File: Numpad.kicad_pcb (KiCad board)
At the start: 2 copper layers, 94 x 162.6 mm, 68 parts, among them J1 SWD, J2 USB_C_Receptacle_USB2.0, SW1 SW_Push, SW10 SW_Push, SW11 SW_Push, SW12 SW_Push, SW13 SW_Push, SW14 SW_Push, SW15 SW_Push, SW16 SW_Push, SW17 SW_Push, SW18 SW_Push, SW19 SW_Push, SW2 SW_Push, SW20 SW_Push, SW21 SW_Push, SW3 SW_Push, SW4 SW_Push, SW5 SW_Push, SW6 SW_Push, SW7 SW_Push, SW8 SW_Push, SW9 SW_Push, U1 SRV05-4, U2 STM32F103C8Tx, U3 XC6206PxxxMR, Y1 8MHz

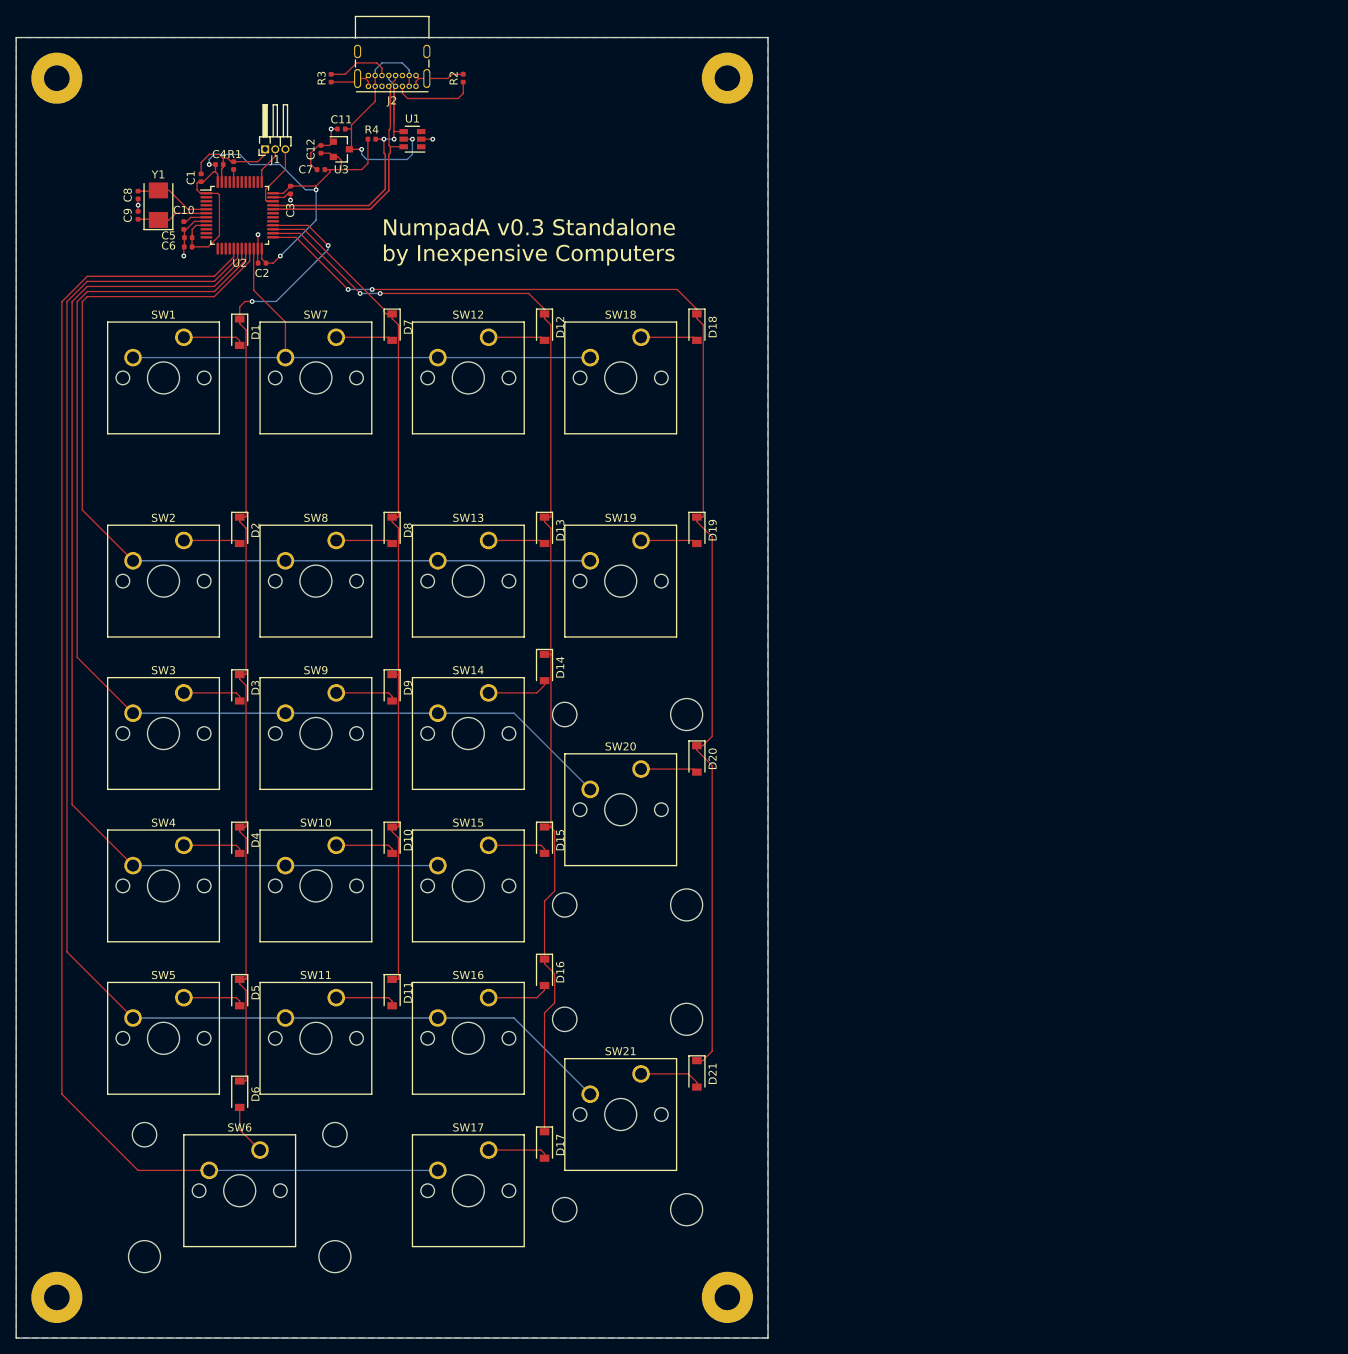
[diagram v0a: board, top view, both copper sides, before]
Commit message: v0.4
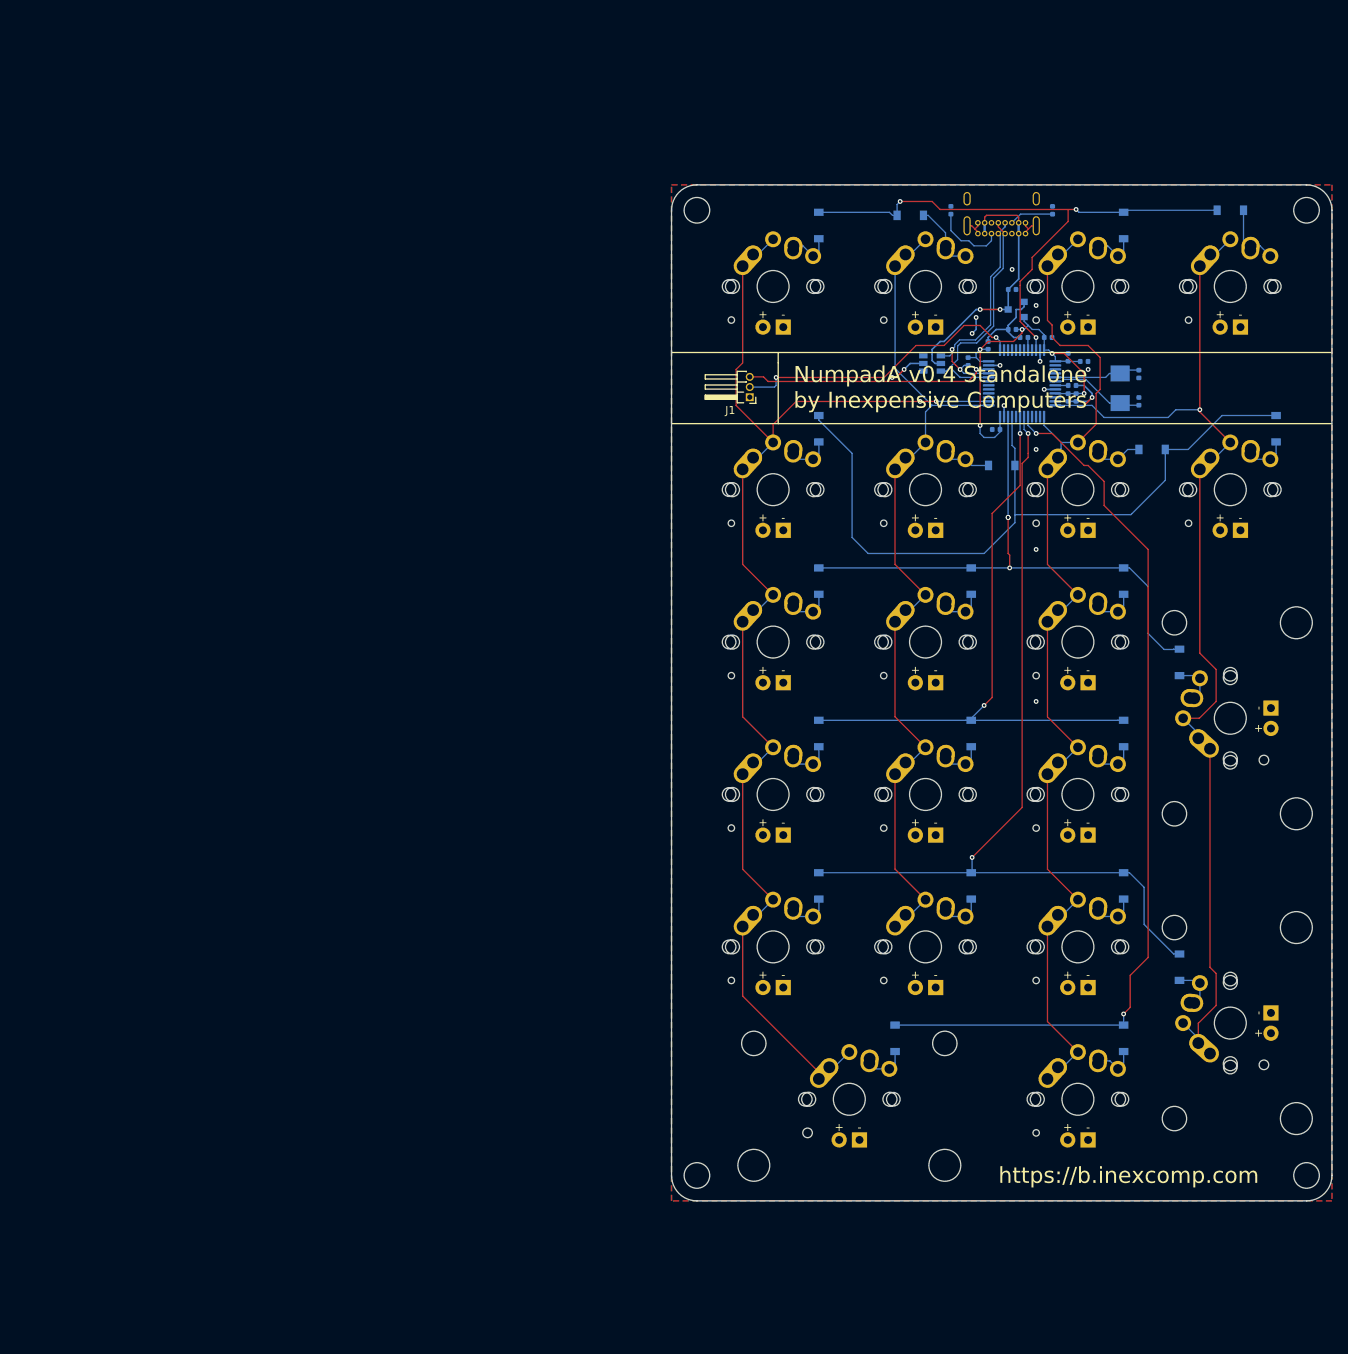
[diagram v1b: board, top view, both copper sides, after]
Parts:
- removed D1, D10, D11, D12, D13, D14, D15, D16, D17, D18, D19, D2, D20, D21, D3, D4, D5, D6, D7, D8, D9: 1N4148, Diode_SMD:D_SOD-123
- removed SW1, SW10, SW11, SW12, SW13, SW14, SW15, SW16, SW17, SW18, SW19, SW2, SW3, SW4, SW5, SW7, SW8, SW9: SW_Push, Button_Switch_Keyboard:SW_Cherry_MX_1.00u_PCB
- removed SW20, SW21: SW_Push, Button_Switch_Keyboard:SW_Cherry_MX_2.00u_Vertical_PCB
- removed SW6: SW_Push, Button_Switch_Keyboard:SW_Cherry_MX_2.00u_PCB
- added D_0: 1N4148, Diode_SMD:D_SOD-123, B.Cu at (126.4, 141.6)
- added D_1: 1N4148, Diode_SMD:D_SOD-123, B.Cu at (116.8, 122.6)
- added D_2: 1N4148, Diode_SMD:D_SOD-123, B.Cu at (135.9, 122.6)
- added D_3: 1N4148, Diode_SMD:D_SOD-123, B.Cu at (154.9, 122.6)
- added D_4: 1N4148, Diode_SMD:D_SOD-123, B.Cu at (116.8, 103.5)
- added D_5: 1N4148, Diode_SMD:D_SOD-123, B.Cu at (135.9, 103.5)
- added D_6: 1N4148, Diode_SMD:D_SOD-123, B.Cu at (154.9, 103.5)
- added D_7: 1N4148, Diode_SMD:D_SOD-123, B.Cu at (116.8, 84.5)
- added D_8: 1N4148, Diode_SMD:D_SOD-123, B.Cu at (135.9, 84.5)
- added D_9: 1N4148, Diode_SMD:D_SOD-123, B.Cu at (154.9, 84.5)
- added D_BKSP1: 1N4148, Diode_SMD:D_SOD-123, B.Cu at (168.3, 38.1)
- added D_DOT1: 1N4148, Diode_SMD:D_SOD-123, B.Cu at (154.9, 141.6)
- added D_ENTER1: 1N4148, Diode_SMD:D_SOD-123, B.Cu at (161.9, 132.7)
- added D_ESC1: 1N4148, Diode_SMD:D_SOD-123, B.Cu at (116.8, 40.0)
- added D_FN1: 1N4148, Diode_SMD:D_SOD-123, B.Cu at (154.9, 40.0)
- added D_MINUS1: 1N4148, Diode_SMD:D_SOD-123, B.Cu at (174.0, 65.4)
- added D_NUMLK1: 1N4148, Diode_SMD:D_SOD-123, B.Cu at (116.8, 65.4)
- added D_PLUS1: 1N4148, Diode_SMD:D_SOD-123, B.Cu at (161.9, 94.6)
- added D_SLASH1: 1N4148, Diode_SMD:D_SOD-123, B.Cu at (139.7, 70.0)
- added D_STAR1: 1N4148, Diode_SMD:D_SOD-123, B.Cu at (158.5, 68.0)
- added D_TAB1: 1N4148, Diode_SMD:D_SOD-123, B.Cu at (128.3, 38.7)
- added SW_0: SW_Push, Keebio-Parts:MX-Alps-Choc-2U, F.Cu at (120.7, 149.2)
- added SW_1: SW_Push, Keebio-Parts:MX-Alps-Choc-1U, F.Cu at (111.1, 130.2)
- added SW_2: SW_Push, Keebio-Parts:MX-Alps-Choc-1U, F.Cu at (130.2, 130.2)
- added SW_3: SW_Push, Keebio-Parts:MX-Alps-Choc-1U, F.Cu at (149.2, 130.2)
- added SW_4: SW_Push, Keebio-Parts:MX-Alps-Choc-1U, F.Cu at (111.1, 111.1)
- added SW_5: SW_Push, Keebio-Parts:MX-Alps-Choc-1U, F.Cu at (130.2, 111.1)
- added SW_6: SW_Push, Keebio-Parts:MX-Alps-Choc-1U, F.Cu at (149.2, 111.1)
- added SW_7: SW_Push, Keebio-Parts:MX-Alps-Choc-1U, F.Cu at (111.1, 92.1)
- added SW_8: SW_Push, Keebio-Parts:MX-Alps-Choc-1U, F.Cu at (130.2, 92.1)
- added SW_9: SW_Push, Keebio-Parts:MX-Alps-Choc-1U, F.Cu at (149.2, 92.1)
- added SW_BKSP1: SW_Push, Keebio-Parts:MX-Alps-Choc-1U, F.Cu at (168.3, 47.6)
- added SW_DOT1: SW_Push, Keebio-Parts:MX-Alps-Choc-1U, F.Cu at (149.2, 149.2)
- added SW_ENTER1: SW_Push, Keebio-Parts:MX-Alps-Choc-2U, F.Cu at (168.3, 139.7)
- added SW_ESC1: SW_Push, Keebio-Parts:MX-Alps-Choc-1U, F.Cu at (111.1, 47.6)
- added SW_FN1: SW_Push, Keebio-Parts:MX-Alps-Choc-1U, F.Cu at (149.2, 47.6)
- added SW_MINUS1: SW_Push, Keebio-Parts:MX-Alps-Choc-1U, F.Cu at (168.3, 73.0)
- added SW_NUMLK1: SW_Push, Keebio-Parts:MX-Alps-Choc-1U, F.Cu at (111.1, 73.0)
- added SW_PLUS1: SW_Push, Keebio-Parts:MX-Alps-Choc-2U, F.Cu at (168.3, 101.6)
- added SW_SLASH1: SW_Push, Keebio-Parts:MX-Alps-Choc-1U, F.Cu at (130.2, 73.0)
- added SW_STAR1: SW_Push, Keebio-Parts:MX-Alps-Choc-1U, F.Cu at (149.2, 73.0)
- added SW_TAB1: SW_Push, Keebio-Parts:MX-Alps-Choc-1U, F.Cu at (130.2, 47.6)
- C1, C10, C11, C12, C2, C3, C4, C5, C6, C7, C8, C9, J2, R1, R2, R3, R4, U1, U2, U3, Y1: moved to B.Cu
- H1, H2, H3, H4: value MountingHole_Pad -> MountingHole; footprint MountingHole:MountingHole_3.2mm_M3_Pad -> MountingHole:MountingHole_3.2mm_M3
- moved C9 127.2 mm to (156.8, 62.0)
- moved C8 127.1 mm to (156.8, 58.6)
- moved Y1 122.4 mm to (154.5, 60.4)
- moved C10 112.8 mm to (148.5, 60.0), turned to 180 degrees
- moved C5 112.8 mm to (149.0, 61.5), turned to 90 degrees
- moved C6 111.6 mm to (148.0, 61.5), turned to 90 degrees
- moved C1 110.7 mm to (148.0, 56.5)
- moved C4 105.8 mm to (145.5, 54.0)
- moved R1 101.1 mm to (142.5, 54.0), turned to 180 degrees
- moved U2 100.0 mm to (142.2, 59.7), turned to 180 degrees
- moved C7 98.4 mm to (150.0, 57.0), turned to 180 degrees
- moved C2 94.1 mm to (139.0, 65.5)
- moved R3 91.7 mm to (146.1, 38.1), turned to 270 degrees
- moved C3 89.3 mm to (138.0, 55.0), turned to 270 degrees
- moved C12 89.3 mm to (141.0, 53.0), turned to 180 degrees
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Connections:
- H1 pad 1: GND -> (no net)
- H2 pad 1: GND -> (no net)
- H3 pad 1: GND -> (no net)
- H4 pad 1: GND -> (no net)
- J2 pad A8: Net-(J2-PadA8) -> (no net)
- J2 pad B8: Net-(J2-PadB8) -> (no net)
- U1 pad 1: Net-(U1-Pad1) -> (no net)
- U1 pad 3: Net-(U1-Pad3) -> (no net)
- U2 pad 10: Net-(U2-Pad10) -> (no net)
- U2 pad 11: Net-(U2-Pad11) -> (no net)
- U2 pad 12: Net-(U2-Pad12) -> col4
- U2 pad 13: Net-(U2-Pad13) -> col3
- U2 pad 14: Net-(U2-Pad14) -> (no net)
- U2 pad 15: Net-(U2-Pad15) -> (no net)
- U2 pad 16: Net-(U2-Pad16) -> (no net)
- U2 pad 2: Net-(U2-Pad2) -> (no net)
- U2 pad 20: row3 -> (no net)
- U2 pad 22: row1 -> row3
- U2 pad 25: col4 -> col2
- U2 pad 26: col3 -> col1
- U2 pad 27: col2 -> (no net)
- U2 pad 28: col1 -> (no net)
- U2 pad 29: Net-(U2-Pad29) -> (no net)
- U2 pad 3: Net-(U2-Pad3) -> (no net)
- U2 pad 30: Net-(U2-Pad30) -> (no net)
- U2 pad 31: Net-(U2-Pad31) -> (no net)
- U2 pad 38: Net-(U2-Pad38) -> (no net)
- U2 pad 39: Net-(U2-Pad39) -> (no net)
- U2 pad 4: Net-(U2-Pad4) -> (no net)
- U2 pad 40: Net-(U2-Pad40) -> (no net)
- U2 pad 41: Net-(U2-Pad41) -> (no net)
- U2 pad 42: Net-(U2-Pad42) -> (no net)
- U2 pad 43: Net-(U2-Pad43) -> (no net)
- U2 pad 45: Net-(U2-Pad45) -> (no net)
- U2 pad 46: Net-(U2-Pad46) -> row1
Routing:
- net row3: track 140.1 -> 71.8 mm, vias 0 -> 3
- net row5: track 178.8 -> 112.2 mm, vias 0 -> 2
- net row6: track 174.8 -> 113.6 mm, vias 0 -> 2
- net row4: track 136.5 -> 78.6 mm, vias 0 -> 2
- net Net-(J1-Pad2): track 4.79 -> 37.0 mm, vias 0 -> 2
- net col4: track 156.5 -> 128.7 mm, vias 2 -> 1
- net VBAT: track 75.9 -> 51.0 mm, vias 3 -> 5
- net col3: track 145.4 -> 120.6 mm, vias 2 -> 0
- net col1: track 124.7 -> 149.2 mm
- net row2: track 116.8 -> 93.2 mm
- net Net-(J1-Pad3): track 9.18 -> 31.0 mm, vias 0 -> 1
- net GND: track 54.2 -> 35.8 mm, vias 6 -> 15
- net Net-(D_TAB1-Pad2): track 0.00 -> 8.66 mm
- net Net-(D_BKSP1-Pad2): track 0.00 -> 8.37 mm
- net Net-(D21-Pad2): track 8.01 -> 0.00 mm
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- added copper zone on F.Cu, net GND
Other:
- board size 94 x 162.6 mm -> 82.6 x 127 mm
- net class Power added: clearance 0.127, trace_width 0.2, via_dia 0.6, via_drill 0.3
- board text added: "NumpadA v0.4 Standalone by Inexpensive Computers"
- board text added: "https://b.inexcomp.com"
- board text removed: "NumpadA v0.3 Standalone by Inexpensive Computers"
